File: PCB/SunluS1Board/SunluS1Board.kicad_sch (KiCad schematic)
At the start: 2 parts, among them U1 STM32C011F4Px

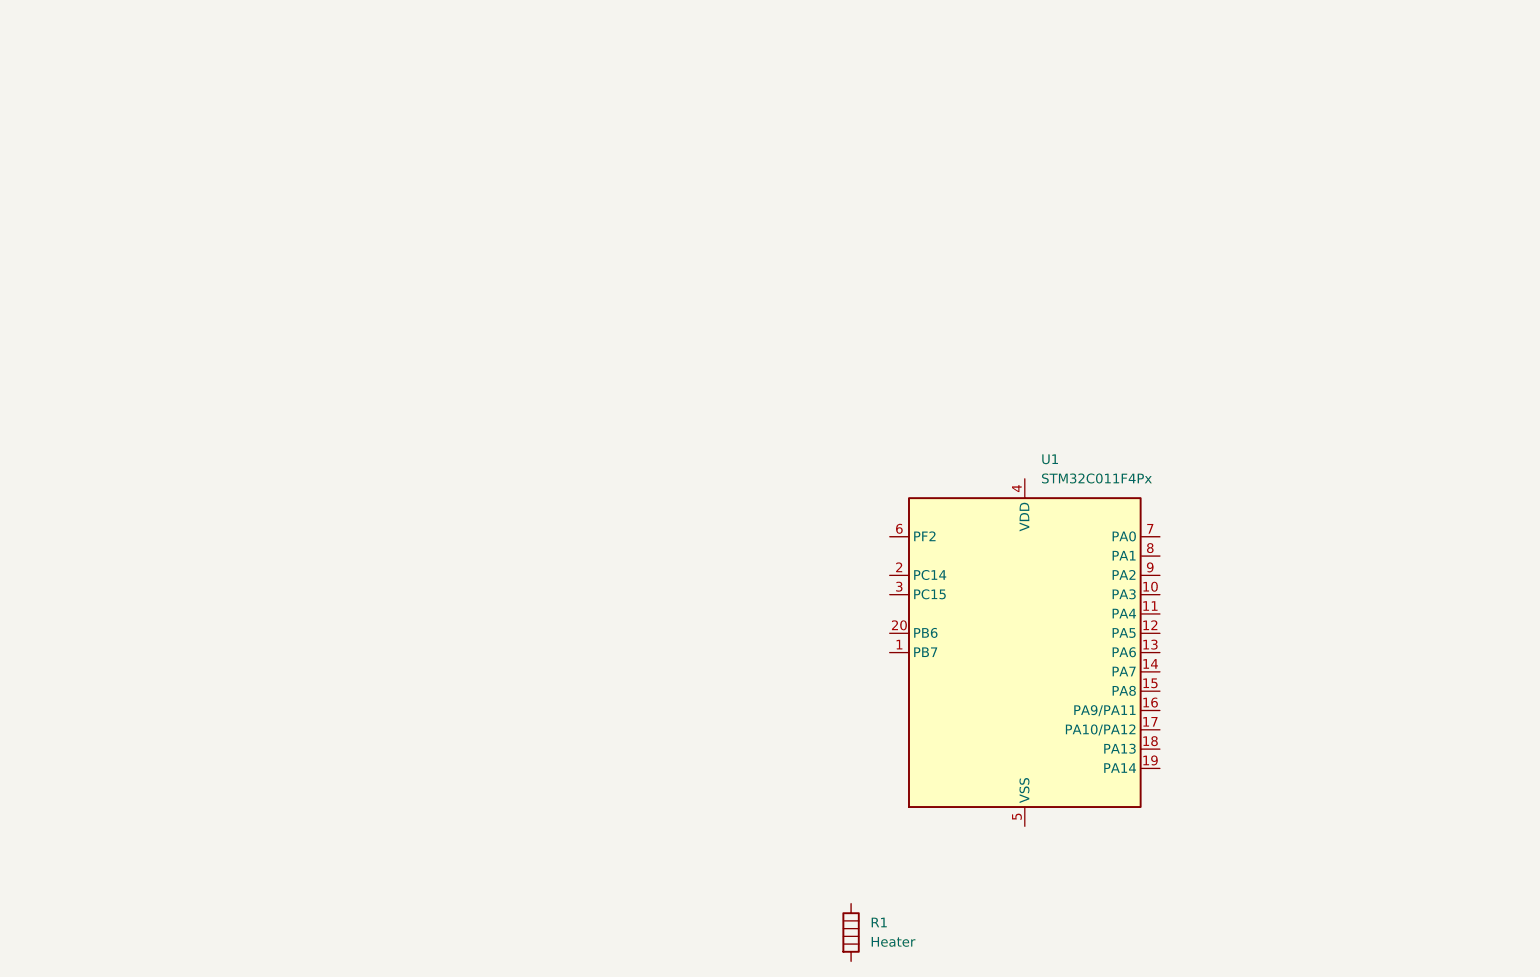
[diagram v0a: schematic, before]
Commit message: start base schematic
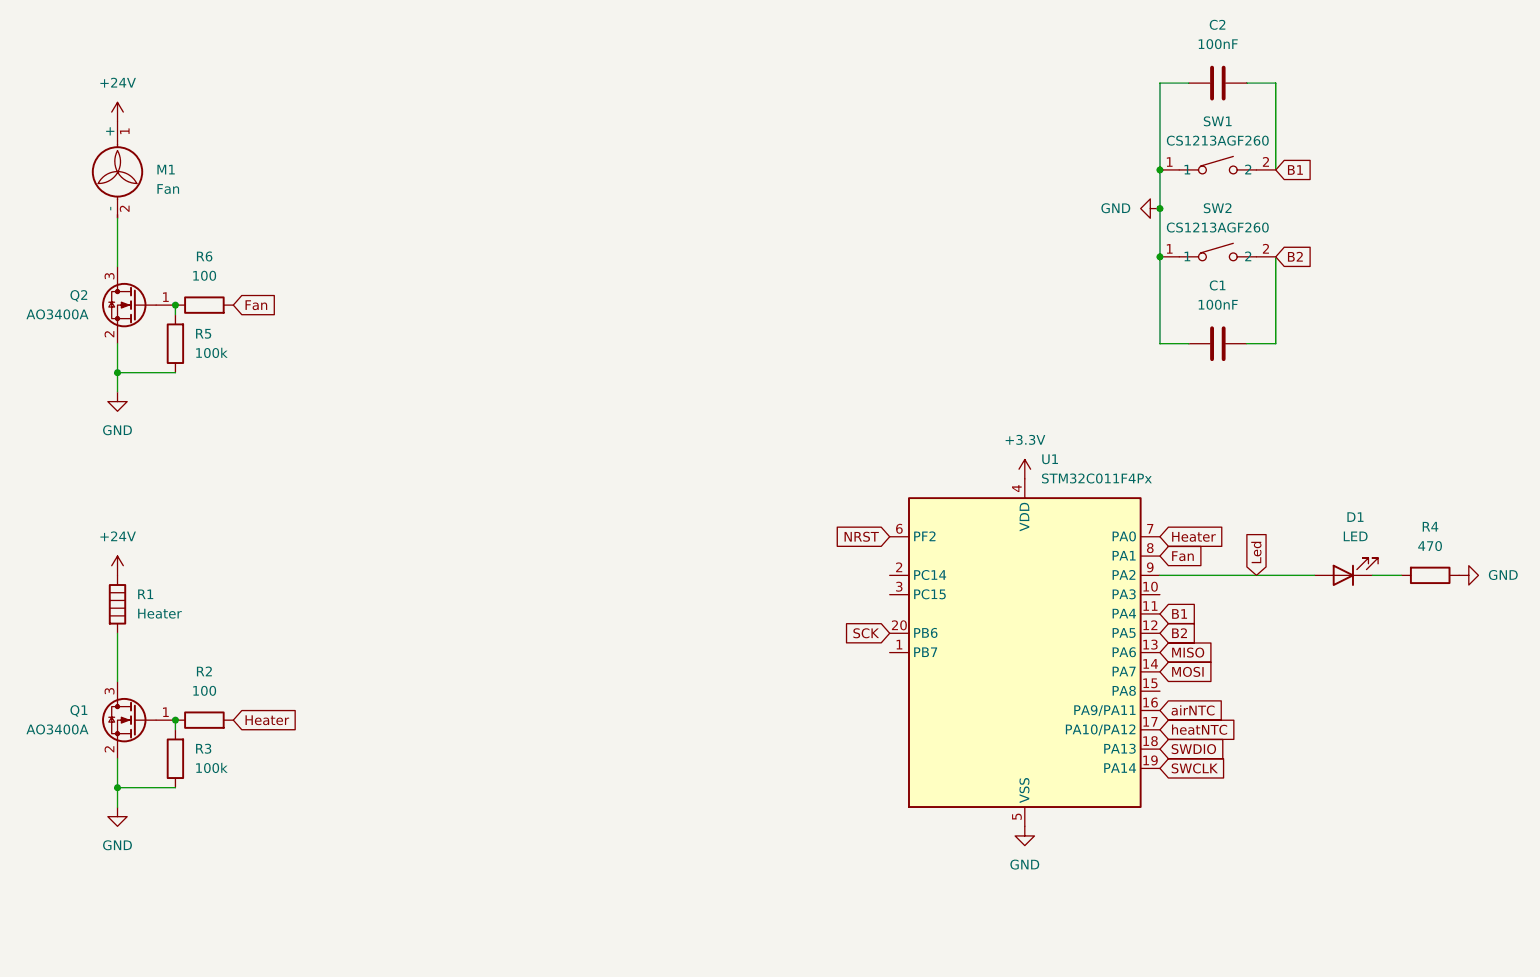
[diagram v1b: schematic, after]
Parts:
- added C1, C2: 100nF, symbol Device:C
- added D1: LED, symbol Device:LED
- added M1: Fan, symbol Motor:Fan
- added Q1, Q2: AO3400A, Package_TO_SOT_SMD:SOT-23, symbol Transistor_FET:AO3400A
- added R2, R6: 100, symbol Device:R
- added R3, R5: 100k, symbol Device:R
- added R4: 470, symbol Device:R
- added SW1, SW2: CS1213AGF260, easyeda2kicad:SW-SMD_L3.9-W3.0-P4.45, symbol easyeda2kicad:TS-1088-AR02016
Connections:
- net +24V: now reaches R1.1
- net +24V: now also M1.1 (+)
- net at R1.2: now also Q1.3 (D)
- net B1: now reaches U1.11 (PA4)
- net B1: now also C2.1, SW1.2
- net B2: now reaches U1.12 (PA5)
- net B2: now also C1.1, SW2.2
- net MISO: now reaches U1.13 (PA6)
- net MOSI: now reaches U1.14 (PA7)
- net airNTC: now reaches U1.16 (PA9/PA11)
- net heatNTC: now reaches U1.17 (PA10/PA12)
- net SWDIO: now reaches U1.18 (PA13)
- net SWCLK: now reaches U1.19 (PA14)
- net SCK: now reaches U1.20 (PB6)
- net +3.3V: now reaches U1.4 (VDD)
- net GND: now reaches U1.5 (VSS)
- net GND: now also C1.2, C2.2, Q1.2 (S), Q2.2 (S), R3.1, R4.1, R5.1, SW1.1, SW2.1
- net NRST: now reaches U1.6 (PF2)
- net Heater: now reaches U1.7 (PA0)
- net Heater: now also R2.2
- net Fan: now reaches U1.8 (PA1)
- net Fan: now also R6.2
- net Led: now reaches U1.9 (PA2)
- net Led: now also D1.2 (A)
- new net: Q1.1 (G), R2.1, R3.2
- new net: D1.1 (K), R4.2
- new net: M1.2 (-), Q2.3 (D)
- new net: Q2.1 (G), R5.2, R6.1
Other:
- moved on the sheet: R1
